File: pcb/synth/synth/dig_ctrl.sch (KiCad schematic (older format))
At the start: 2 parts, among them U12 PCF8574A, U13 AD5694R

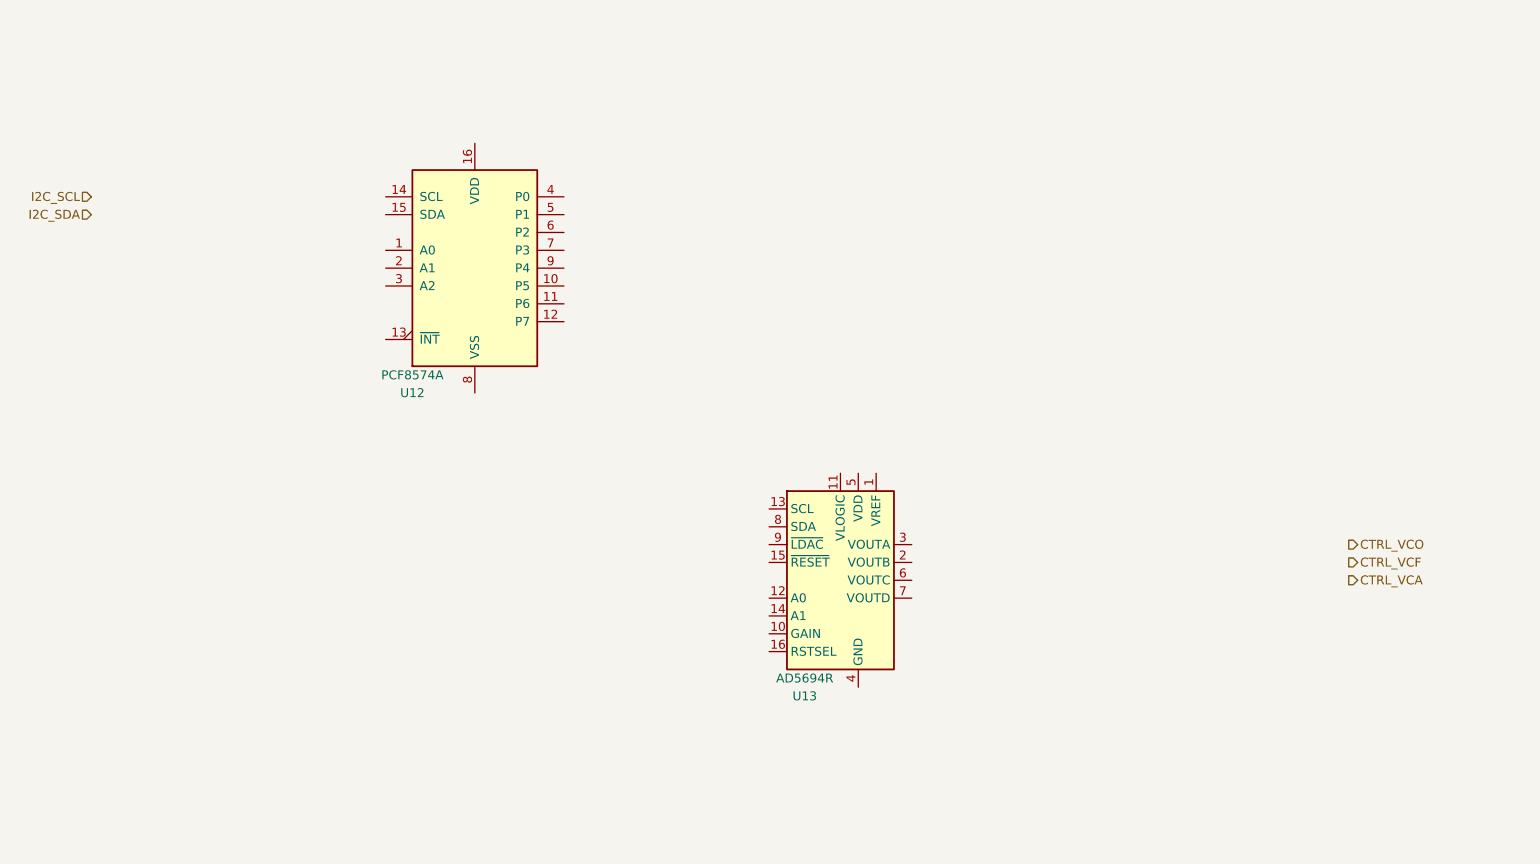
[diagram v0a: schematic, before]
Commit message: inital synth schematic
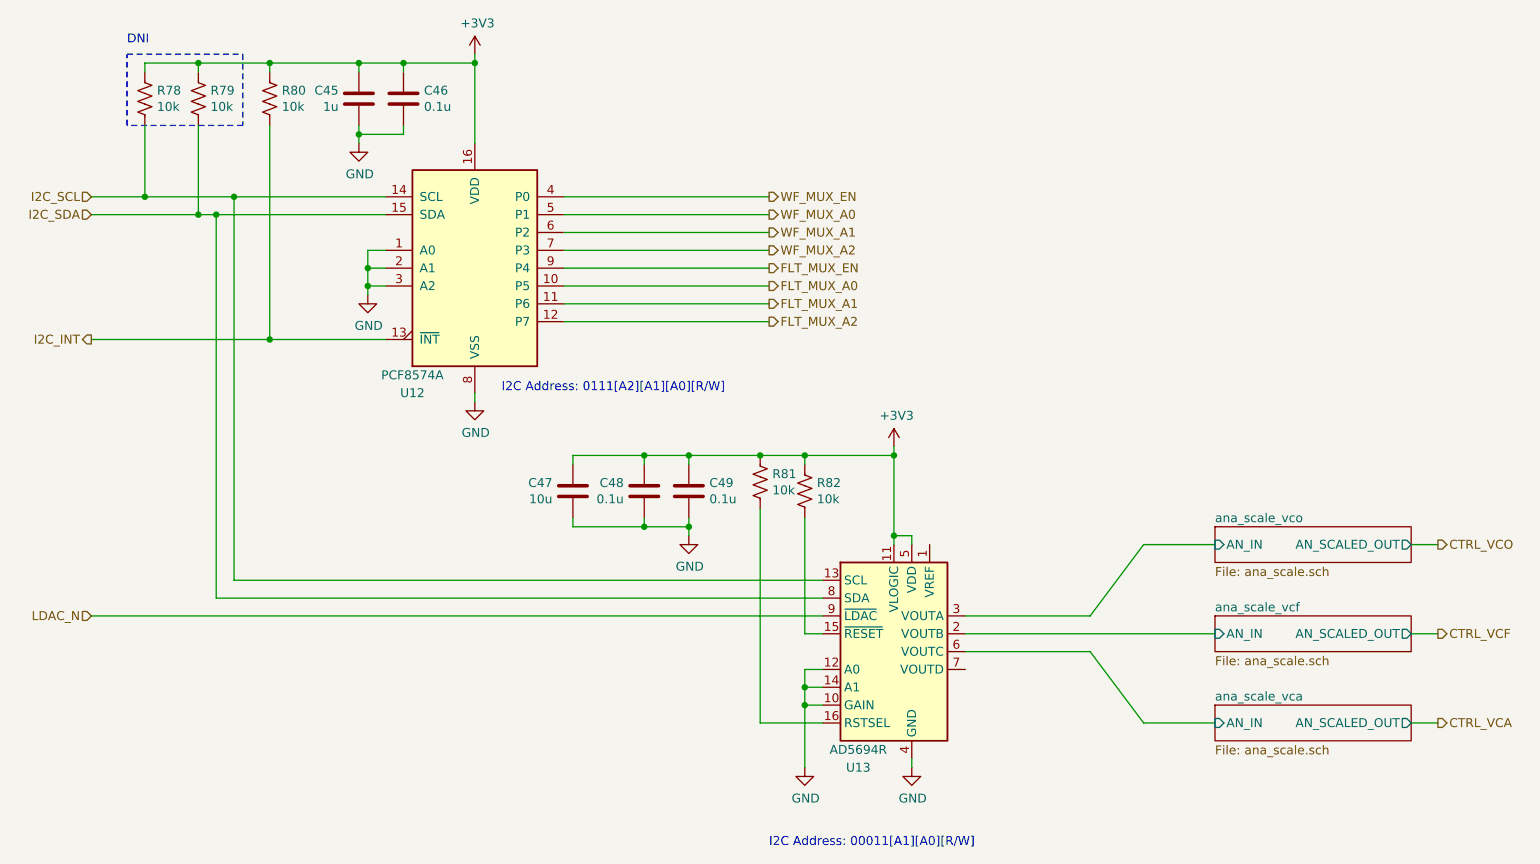
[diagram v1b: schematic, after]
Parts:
- added C45: 1u, Capacitor_SMD:C_0603_1608Metric_Pad1.05x0.95mm_HandSolder, symbol Device:C
- added C46, C48, C49: 0.1u, Capacitor_SMD:C_0603_1608Metric_Pad1.05x0.95mm_HandSolder, symbol Device:C
- added C47: 10u, Capacitor_SMD:C_0603_1608Metric_Pad1.05x0.95mm_HandSolder, symbol Device:C
- added R78, R79, R80, R81, R82: 10k, Resistor_SMD:R_0603_1608Metric_Pad1.05x0.95mm_HandSolder, symbol Device:R_US
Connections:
- net I2C_SCL: now also U12.14 (SCL), U13.13 (SCL), R78.2
- net I2C_SDA: now also U12.15 (SDA), U13.8 (SDA), R79.2
- net GND: now reaches U12.1 (A0)
- net GND: now also U12.2 (A1), U12.3 (A2), U12.8 (VSS), U13.10 (GAIN), U13.12 (A0), U13.14 (A1), U13.4 (GND), C45.2, C46.2, C47.2, C48.2, C49.2
- net FLT_MUX_A0: now reaches U12.10 (P5)
- net FLT_MUX_A1: now reaches U12.11 (P6)
- net FLT_MUX_A2: now reaches U12.12 (P7)
- net I2C_INT: now reaches U12.13 (~INT~)
- net I2C_INT: now also R80.2
- net +3V3: now reaches U12.16 (VDD)
- net +3V3: now also U13.11 (VLOGIC), U13.5 (VDD), C45.1, C46.1, C47.1, C48.1, C49.1, R78.1, R79.1, R80.1, R81.1, R82.1
- net WF_MUX_EN: now reaches U12.4 (P0)
- net WF_MUX_A0: now reaches U12.5 (P1)
- net WF_MUX_A1: now reaches U12.6 (P2)
- net WF_MUX_A2: now reaches U12.7 (P3)
- net FLT_MUX_EN: now reaches U12.9 (P4)
- net at U13.15 (~RESET): now also R82.2
- net at U13.16 (RSTSEL): now also R81.2
- net ana_scale_vcf/AN_IN: now reaches U13.2 (VOUTB)
- net ana_scale_vco/AN_IN: now reaches U13.3 (VOUTA)
- net ana_scale_vca/AN_IN: now reaches U13.6 (VOUTC)
- net LDAC_N: now reaches U13.9 (~LDAC)
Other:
- note added: "DNI"
- note added: "I2C Address: 00011[A1][A0][R/W]"
- note added: "I2C Address: 0111[A2][A1][A0][R/W]"
- moved on the sheet: U13
